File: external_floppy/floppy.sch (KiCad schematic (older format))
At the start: 8 parts, among them J1 12VDC, J2 FLOPPY_PWR, J3 DATA_IN, J4 FLOPPY, U1 L7805

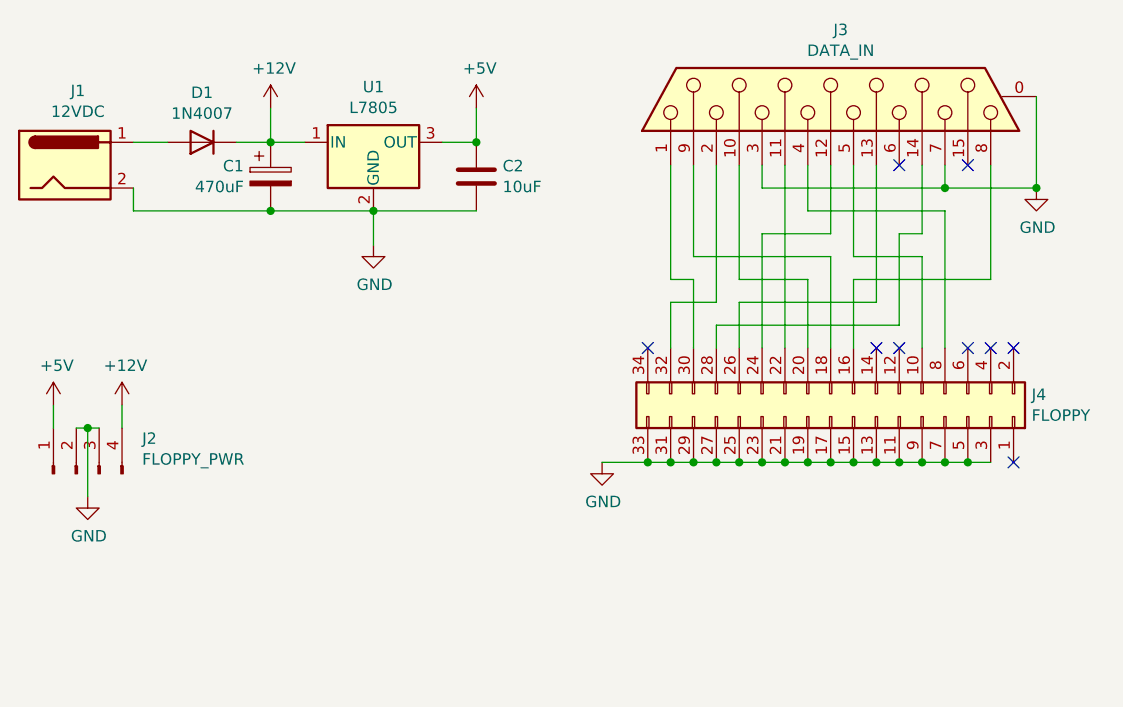
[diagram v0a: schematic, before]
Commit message: a
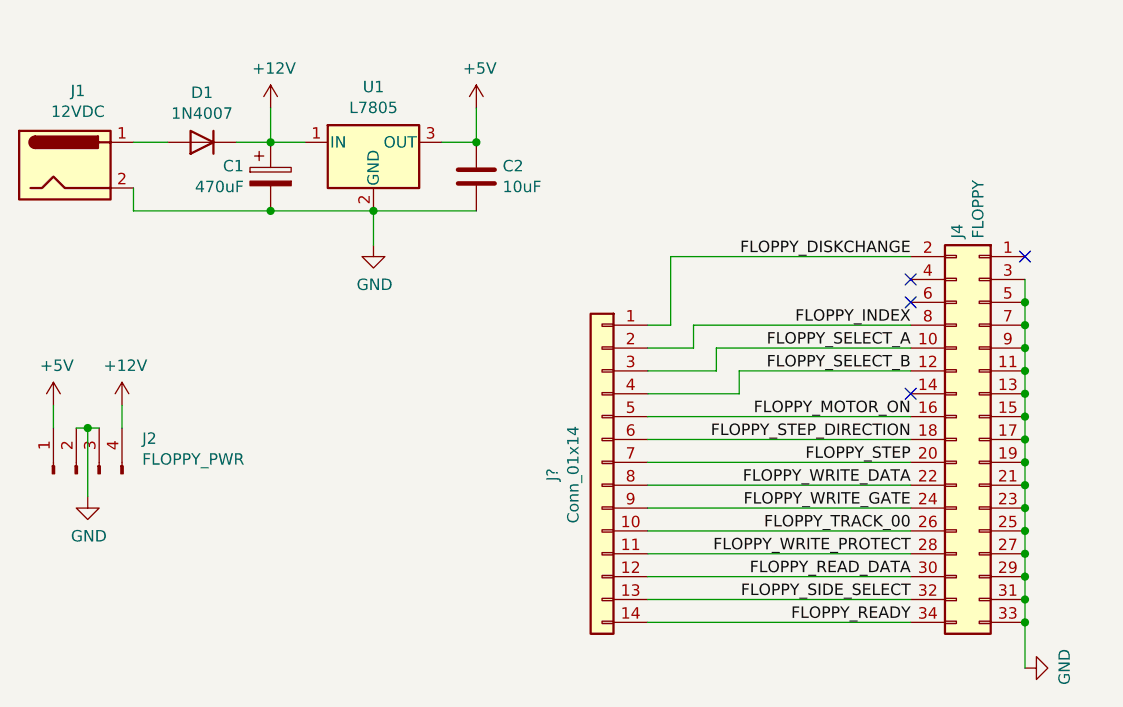
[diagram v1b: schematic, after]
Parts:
- removed J3: DATA_IN, Connector_Dsub:DSUB-15_Female_Horizontal_P2.77x2.84mm_EdgePinOffset4.94mm_Housed_MountingHolesOffset7.48mm, symbol Connector:DB15_Female_MountingHoles
- added J?: Conn_01x14, symbol Connector_Generic:Conn_01x14
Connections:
- net FLOPPY_READ_DATA: now reaches J4.30 (Pin_30)
- net FLOPPY_READ_DATA: now also J?.12 (Pin_12)
- net FLOPPY_STEP: now reaches J4.20 (Pin_20)
- net FLOPPY_STEP: now also J?.7 (Pin_7)
- net FLOPPY_WRITE_DATA: now reaches J4.22 (Pin_22)
- net FLOPPY_WRITE_DATA: now also J?.8 (Pin_8)
- net FLOPPY_WRITE_GATE: now reaches J4.24 (Pin_24)
- net FLOPPY_WRITE_GATE: now also J?.9 (Pin_9)
- net FLOPPY_TRACK_00: now reaches J4.26 (Pin_26)
- net FLOPPY_TRACK_00: now also J?.10 (Pin_10)
- net FLOPPY_WRITE_PROTECT: now reaches J4.28 (Pin_28)
- net FLOPPY_WRITE_PROTECT: now also J?.11 (Pin_11)
- net FLOPPY_SIDE_SELECT: now reaches J4.32 (Pin_32)
- net FLOPPY_SIDE_SELECT: now also J?.13 (Pin_13)
- net FLOPPY_INDEX: now reaches J4.8 (Pin_8)
- net FLOPPY_INDEX: now also J?.2 (Pin_2)
- net FLOPPY_SELECT_A: now reaches J4.10 (Pin_10)
- net FLOPPY_SELECT_A: now also J?.3 (Pin_3)
- net FLOPPY_MOTOR_ON: now reaches J4.16 (Pin_16)
- net FLOPPY_MOTOR_ON: now also J?.5 (Pin_5)
- net FLOPPY_STEP_DIRECTION: now reaches J4.18 (Pin_18)
- net FLOPPY_STEP_DIRECTION: now also J?.6 (Pin_6)
- net FLOPPY_SELECT_B: now reaches J4.12 (Pin_12)
- net FLOPPY_SELECT_B: now also J?.4 (Pin_4)
- net FLOPPY_DISKCHANGE: now reaches J4.2 (Pin_2)
- net FLOPPY_DISKCHANGE: now also J?.1 (Pin_1)
- net FLOPPY_READY: now reaches J4.34 (Pin_34)
- net FLOPPY_READY: now also J?.14 (Pin_14)
- no-connect marks 9 -> 4
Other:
- moved on the sheet: J4
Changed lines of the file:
@@
 	1    0    0    -1
-$EndComp
-$Comp
-L Connector:DB15_Female_MountingHoles J3
-U 1 1 5FC416BA
-P 4450 1050
-F 0 "J3" V 4742 1006 50  0000 C CNN
-F 1 "DATA_IN" V 4651 1006 50  0000 C CNN
-F 2 "Connector_Dsub:DSUB-15_Female_Horizontal_P2.77x2.84mm_EdgePinOffset4.94mm_Housed_MountingHolesOffset7.48mm" H 4450 1050 50  0001 C CNN
-F 3 " ~" H 4450 1050 50  0001 C CNN
-	1    4450 1050
-	0    -1   -1   0
-$EndComp
-$Comp
-L Connector_Generic:Conn_02x17_Odd_Even J4
-U 1 1 5FC468F3
-P 4450 2450
-F 0 "J4" V 4546 3329 50  0000 L CNN
-F 1 "FLOPPY" V 4455 3329 50  0000 L CNN
-F 2 "Connector_PinHeader_2.54mm:PinHeader_2x17_P2.54mm_Horizontal" H 4450 2450 50  0001 C CNN
-F 3 "~" H 4450 2450 50  0001 C CNN
-	1    4450 2450
-	0    1    -1   0
 $EndComp
 Wire Wire Line
@@
 	1050 2500 1050 2400
 $Comp
-L power:GND #PWR08
-U 1 1 5FC5A5CD
-P 5350 1450
-F 0 "#PWR08" H 5350 1200 50  0001 C CNN
-F 1 "GND" H 5355 1277 50  0000 C CNN
-F 2 "" H 5350 1450 50  0001 C CNN
-F 3 "" H 5350 1450 50  0001 C CNN
-	1    5350 1450
-	1    0    0    -1
-$EndComp
-$Comp
 L power:GND #PWR07
 U 1 1 5FC5B179
+P 5300 3550
+F 0 "#PWR07" H 5300 3300 50  0001 C CNN
+F 1 "GND" H 5305 3377 50  0000 C CNN
+F 2 "" H 5300 3550 50  0001 C CNN
+F 3 "" H 5300 3550 50  0001 C CNN
+	1    5300 3550
+	0    -1   -1   0
+$EndComp
+NoConn ~ 5300 1750
+NoConn ~ 4800 1850
+NoConn ~ 4800 1950
+NoConn ~ 4800 2350
+Wire Wire Line
+	1400 1250 1550 1250
+Wire Wire Line
+	1400 1550 2000 1550
+Wire Wire Line
+	2900 1100 2900 1250
+Wire Wire Line
+	2000 1250 2000 1100
+Wire Wire Line
+	2450 1550 2450 1700
+$Comp
+L Connector_Generic:Conn_01x14 J?
+U 1 1 5FE91E46
 P 3450 2650
-F 0 "#PWR07" H 3450 2400 50  0001 C CNN
-F 1 "GND" H 3455 2477 50  0000 C CNN
+F 0 "J?" V 3667 2596 50  0000 C CNN
+F 1 "Conn_01x14" V 3576 2596 50  0000 C CNN
 F 2 "" H 3450 2650 50  0001 C CNN
-F 3 "" H 3450 2650 50  0001 C CNN
+F 3 "~" H 3450 2650 50  0001 C CNN
 	1    3450 2650
-	1    0    0    -1
-$EndComp
-NoConn ~ 5050 1350
-Wire Wire Line
-	3450 2650 3650 2650
-Connection ~ 3650 2650
-Wire Wire Line
-	3650 2650 3750 2650
-Connection ~ 3750 2650
-Wire Wire Line
-	3750 2650 3850 2650
-Connection ~ 3850 2650
-Wire Wire Line
-	3850 2650 3950 2650
-Connection ~ 3950 2650
-Wire Wire Line
-	3950 2650 4050 2650
-Connection ~ 4050 2650
-Wire Wire Line
-	4050 2650 4150 2650
-Connection ~ 4150 2650
-Wire Wire Line
-	4150 2650 4250 2650
-Connection ~ 4250 2650
-Wire Wire Line
-	4250 2650 4350 2650
-Connection ~ 4350 2650
-Wire Wire Line
-	4350 2650 4450 2650
-Connection ~ 4450 2650
-Wire Wire Line
-	4450 2650 4550 2650
-Connection ~ 4550 2650
-Wire Wire Line
-	4550 2650 4650 2650
-Connection ~ 4650 2650
-Wire Wire Line
-	4650 2650 4750 2650
-Connection ~ 4750 2650
-Wire Wire Line
-	4750 2650 4850 2650
-Connection ~ 4850 2650
-Wire Wire Line
-	4850 2650 4950 2650
-Connection ~ 4950 2650
-Wire Wire Line
-	4950 2650 5050 2650
-Connection ~ 5050 2650
-Wire Wire Line
-	5050 2650 5150 2650
-NoConn ~ 5250 2650
-NoConn ~ 5250 2150
-Wire Wire Line
-	3750 1350 3750 1850
-Wire Wire Line
-	3750 1850 3850 1850
-Wire Wire Line
-	3850 1850 3850 2150
-Wire Wire Line
-	4450 2150 4450 1750
-Wire Wire Line
-	4450 1750 3850 1750
-Wire Wire Line
-	3850 1750 3850 1350
-Wire Wire Line
-	3750 2150 3750 1950
-Wire Wire Line
-	3750 1950 3950 1950
-Wire Wire Line
-	3950 1950 3950 1350
-Wire Wire Line
-	4350 2150 4350 1850
-Wire Wire Line
-	4350 1850 4050 1850
-Wire Wire Line
-	4050 1850 4050 1350
-Wire Wire Line
-	4250 1350 4250 2150
-Wire Wire Line
-	4950 2150 4950 1550
-Wire Wire Line
-	4950 1550 4350 1550
-Wire Wire Line
-	4350 1550 4350 1350
-Wire Wire Line
-	4450 1350 4450 1650
-Wire Wire Line
-	4450 1650 4150 1650
-Wire Wire Line
-	4150 1650 4150 2150
-Wire Wire Line
-	4850 2150 4850 1750
-Wire Wire Line
-	4850 1750 4550 1750
-Wire Wire Line
-	4550 1750 4550 1350
-Wire Wire Line
-	4050 2150 4050 1950
-Wire Wire Line
-	4050 1950 4650 1950
-Wire Wire Line
-	4650 1950 4650 1350
-NoConn ~ 4750 1350
-Wire Wire Line
-	3950 2150 3950 2050
-Wire Wire Line
-	3950 2050 4750 2050
-Wire Wire Line
-	4750 2050 4750 1650
-Wire Wire Line
-	4750 1650 4850 1650
-Wire Wire Line
-	4850 1650 4850 1350
-Wire Wire Line
-	4550 2150 4550 1850
-Wire Wire Line
-	4550 1850 5150 1850
-Wire Wire Line
-	5150 1850 5150 1350
-Wire Wire Line
-	4150 1350 4150 1450
-Wire Wire Line
-	4150 1450 4950 1450
-Wire Wire Line
-	5350 1450 5350 1050
-Wire Wire Line
-	4950 1350 4950 1450
-Connection ~ 4950 1450
-Wire Wire Line
-	4950 1450 5350 1450
-Connection ~ 5350 1450
-NoConn ~ 5150 2150
-NoConn ~ 5050 2150
-NoConn ~ 4750 2150
-NoConn ~ 4650 2150
-NoConn ~ 3650 2150
-Wire Wire Line
-	1400 1250 1550 1250
-Wire Wire Line
-	1400 1550 2000 1550
-Wire Wire Line
-	2900 1100 2900 1250
-Wire Wire Line
-	2000 1250 2000 1100
-Wire Wire Line
-	2450 1550 2450 1700
+	-1   0    0    -1
+$EndComp
+Wire Wire Line
+	4800 2650 3650 2650
+Wire Wire Line
+	3650 2750 4800 2750
+Wire Wire Line
+	4800 2850 3650 2850
+Wire Wire Line
+	3650 2950 4800 2950
+Wire Wire Line
+	4800 3050 3650 3050
+Wire Wire Line
+	3650 3150 4800 3150
+Wire Wire Line
+	4800 3250 3650 3250
+Connection ~ 5300 2150
+Wire Wire Line
+	5300 2150 5300 2050
+Connection ~ 5300 2050
+Wire Wire Line
+	5300 1950 5300 1850
+Wire Wire Line
+	5300 2050 5300 1950
+Connection ~ 5300 1950
+Wire Wire Line
+	5300 3550 5300 3350
+Connection ~ 5300 3350
+Wire Wire Line
+	5300 3350 5300 3250
+Connection ~ 5300 3250
+Wire Wire Line
+	5300 3250 5300 3150
+Connection ~ 5300 3150
+Wire Wire Line
+	5300 3150 5300 3050
+Connection ~ 5300 3050
+Wire Wire Line
+	5300 3050 5300 2950
+Connection ~ 5300 2950
+Wire Wire Line
+	5300 2950 5300 2850
+Connection ~ 5300 2850
+Wire Wire Line
+	5300 2850 5300 2750
+Connection ~ 5300 2750
+Wire Wire Line
+	5300 2750 5300 2650
+Connection ~ 5300 2650
+Wire Wire Line
+	5300 2650 5300 2550
+Connection ~ 5300 2550
+Wire Wire Line
+	5300 2550 5300 2450
+Connection ~ 5300 2450
+Wire Wire Line
+	5300 2450 5300 2350
+Connection ~ 5300 2350
+Wire Wire Line
+	5300 2250 5300 2150
+Wire Wire Line
+	5300 2350 5300 2250
+Connection ~ 5300 2250
+$Comp
+L Connector_Generic:Conn_02x17_Odd_Even J4
+U 1 1 5FC468F3
+P 5100 2550
+F 0 "J4" V 5196 3429 50  0000 L CNN
+F 1 "FLOPPY" V 5105 3429 50  0000 L CNN
+F 2 "Connector_PinHeader_2.54mm:PinHeader_2x17_P2.54mm_Horizontal" H 5100 2550 50  0001 C CNN
+F 3 "~" H 5100 2550 50  0001 C CNN
+	1    5100 2550
+	-1   0    0    -1
+$EndComp
+Wire Wire Line
+	4800 2550 3650 2550
+Wire Wire Line
+	4800 2450 3650 2450
+Wire Wire Line
+	4800 2250 4050 2250
+Wire Wire Line
+	4050 2250 4050 2350
+Wire Wire Line
+	4050 2350 3650 2350
+Wire Wire Line
+	4800 2150 3950 2150
+Wire Wire Line
+	3950 2150 3950 2250
+Wire Wire Line
+	3950 2250 3650 2250
+Wire Wire Line
+	4800 2050 3850 2050
+Wire Wire Line
+	3850 2050 3850 2150
+Wire Wire Line
+	3850 2150 3650 2150
+Wire Wire Line
+	4800 3350 3650 3350
+Wire Wire Line
+	4800 1750 3750 1750
+Wire Wire Line
+	3750 2050 3650 2050
+Wire Wire Line
+	3750 1750 3750 2050
+Text Label 4800 2050 2    50   ~ 0
+FLOPPY_INDEX
+Text Label 4800 2150 2    50   ~ 0
+FLOPPY_SELECT_A
+Text Label 4800 2250 2    50   ~ 0
+FLOPPY_SELECT_B
+Text Label 4800 2450 2    50   ~ 0
+FLOPPY_MOTOR_ON
+Text Label 4800 2550 2    50   ~ 0
+FLOPPY_STEP_DIRECTION
+Text Label 4800 2650 2    50   ~ 0
+FLOPPY_STEP
+Text Label 4800 2750 2    50   ~ 0
+FLOPPY_WRITE_DATA
+Text Label 4800 2850 2    50   ~ 0
+FLOPPY_WRITE_GATE
+Text Label 4800 2950 2    50   ~ 0
+FLOPPY_TRACK_00
+Text Label 4800 3050 2    50   ~ 0
+FLOPPY_WRITE_PROTECT
+Text Label 4800 3150 2    50   ~ 0
+FLOPPY_READ_DATA
+Text Label 4800 3250 2    50   ~ 0
+FLOPPY_SIDE_SELECT
+Text Label 4800 3350 2    50   ~ 0
+FLOPPY_READY
+Text Label 4800 1750 2    50   ~ 0
+FLOPPY_DISKCHANGE
 $EndSCHEMATC
